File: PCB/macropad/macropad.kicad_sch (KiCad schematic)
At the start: 13 parts, among them SW1 SW_Push, SW10 SW_Push, SW11 SW_Push, SW12 RotaryEncoder_Switch, SW2 SW_Push, SW3 SW_Push, SW4 SW_Push, SW5 SW_Push, SW6 SW_Push, SW7 SW_Push, SW8 SW_Push, SW9 SW_Push, U1 MOUDLE-SEEEDUINO-XIAO

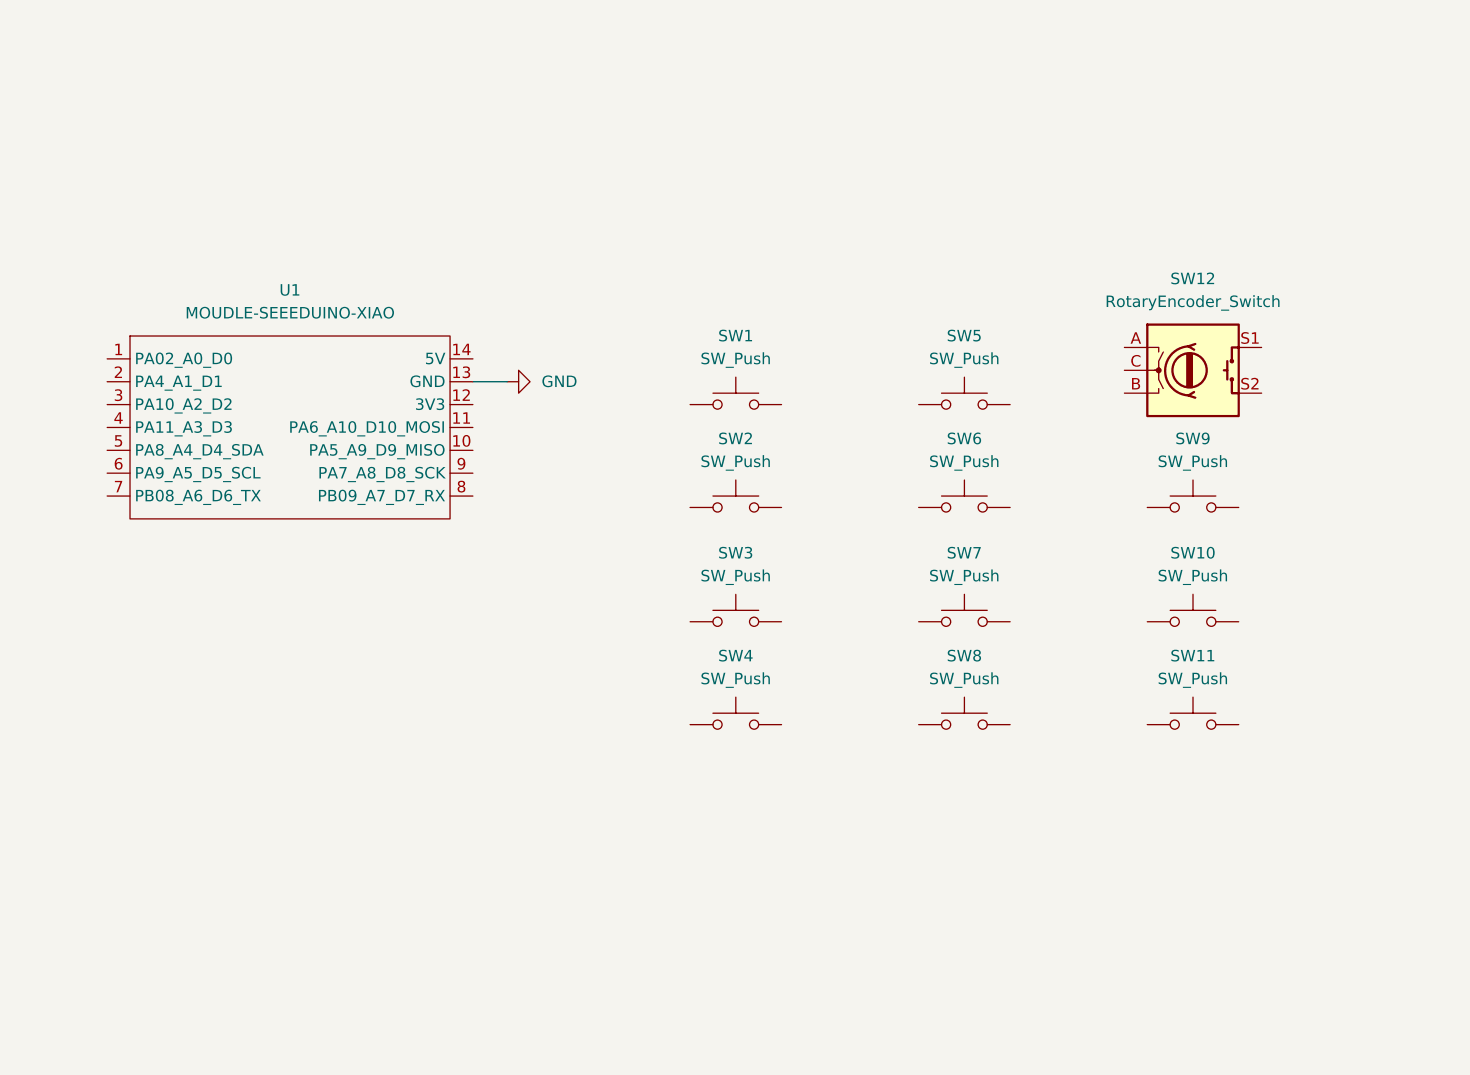
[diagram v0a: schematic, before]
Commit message: Created Basic Schematic and PCB
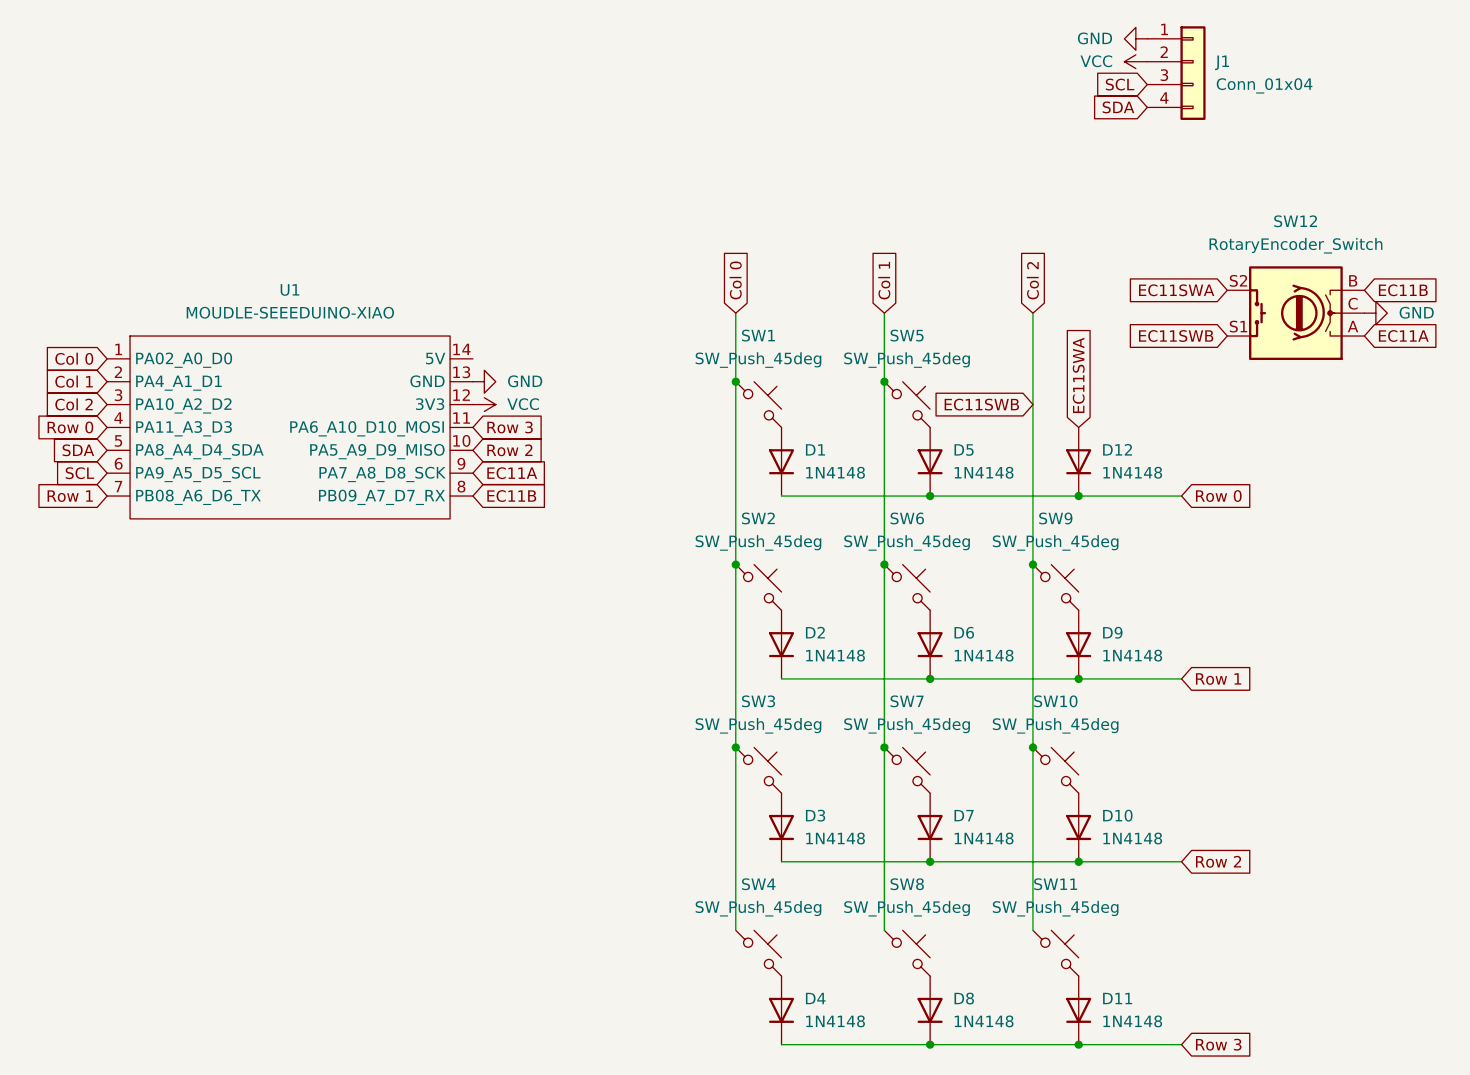
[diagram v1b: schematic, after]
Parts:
- removed SW1, SW10, SW11, SW2, SW3, SW4, SW5, SW6, SW7, SW8, SW9: SW_Push, symbol Switch:SW_Push
- added D1, D10, D11, D12, D2, D3, D4, D5, D6, D7, D8, D9: 1N4148, Diode_THT:D_DO-35_SOD27_P7.62mm_Horizontal, symbol Diode:1N4148
- added J1: Conn_01x04, footprints:SSD1306-0.91-OLED-4pin-128x32, symbol Connector_Generic:Conn_01x04
- added SW1, SW10, SW11, SW2, SW3, SW4, SW5, SW6, SW7, SW8, SW9: SW_Push_45deg, Button_Switch_Keyboard:SW_Cherry_MX_1.00u_PCB, symbol Switch:SW_Push_45deg
- SW12: footprint (none) -> Rotary_Encoder:RotaryEncoder_Alps_EC11E-Switch_Vertical_H20mm
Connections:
- net GND: now also SW12.C, J1.1 (Pin_1)
- net EC11A: now reaches SW12.A
- net EC11A: now also U1.9 (PA7_A8_D8_SCK)
- net EC11B: now reaches SW12.B
- net EC11B: now also U1.8 (PB09_A7_D7_RX)
- net Col 2: now reaches SW12.S1
- net Col 2: now also U1.3 (PA10_A2_D2), SW10.1, SW11.1, SW9.1
- net EC11SWA: now reaches SW12.S2
- net EC11SWA: now also D12.2 (A)
- net Col 0: now reaches U1.1 (PA02_A0_D0)
- net Col 0: now also SW1.1, SW2.1, SW3.1, SW4.1
- net Row 2: now reaches U1.10 (PA5_A9_D9_MISO)
- net Row 2: now also D10.1 (K), D3.1 (K), D7.1 (K)
- net Row 3: now reaches U1.11 (PA6_A10_D10_MOSI)
- net Row 3: now also D11.1 (K), D4.1 (K), D8.1 (K)
- net VCC: now reaches U1.12 (3V3)
- net VCC: now also J1.2 (Pin_2)
- net Col 1: now reaches U1.2 (PA4_A1_D1)
- net Col 1: now also SW5.1, SW6.1, SW7.1, SW8.1
- net Row 0: now reaches U1.4 (PA11_A3_D3)
- net Row 0: now also D1.1 (K), D12.1 (K), D5.1 (K)
- net SDA: now reaches U1.5 (PA8_A4_D4_SDA)
- net SDA: now also J1.4 (Pin_4)
- net SCL: now reaches U1.6 (PA9_A5_D5_SCL)
- net SCL: now also J1.3 (Pin_3)
- net Row 1: now reaches U1.7 (PB08_A6_D6_TX)
- net Row 1: now also D2.1 (K), D6.1 (K), D9.1 (K)
- new net: D4.2 (A), SW4.2
- new net: D2.2 (A), SW2.2
- new net: D6.2 (A), SW6.2
- new net: D5.2 (A), SW5.2
- new net: D1.2 (A), SW1.2
- new net: D8.2 (A), SW8.2
- new net: D10.2 (A), SW10.2
- new net: D7.2 (A), SW7.2
- new net: D3.2 (A), SW3.2
- new net: D11.2 (A), SW11.2
- new net: D9.2 (A), SW9.2
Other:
- moved on the sheet: SW12
